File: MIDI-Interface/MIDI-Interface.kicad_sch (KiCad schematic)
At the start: 65 parts, among them J1 Conn_01x06_Pin, J2 Conn_01x01_Pin, J3 Conn_01x01_Pin, J4 Conn_01x14_Pin, J5 Conn_01x14_Pin, SW1 RotaryEncoder_Switch, U1 TL074, U10 Aux_flush, U11 Aux_flush, U12 Aux_flush, U13 Aux_flush, U2 L7806, U3 EL817, U4 TL072, U5 TL074, U6 Aux_flush, U7 Aux_flush, U8 Aux_flush, U9 Aux_flush

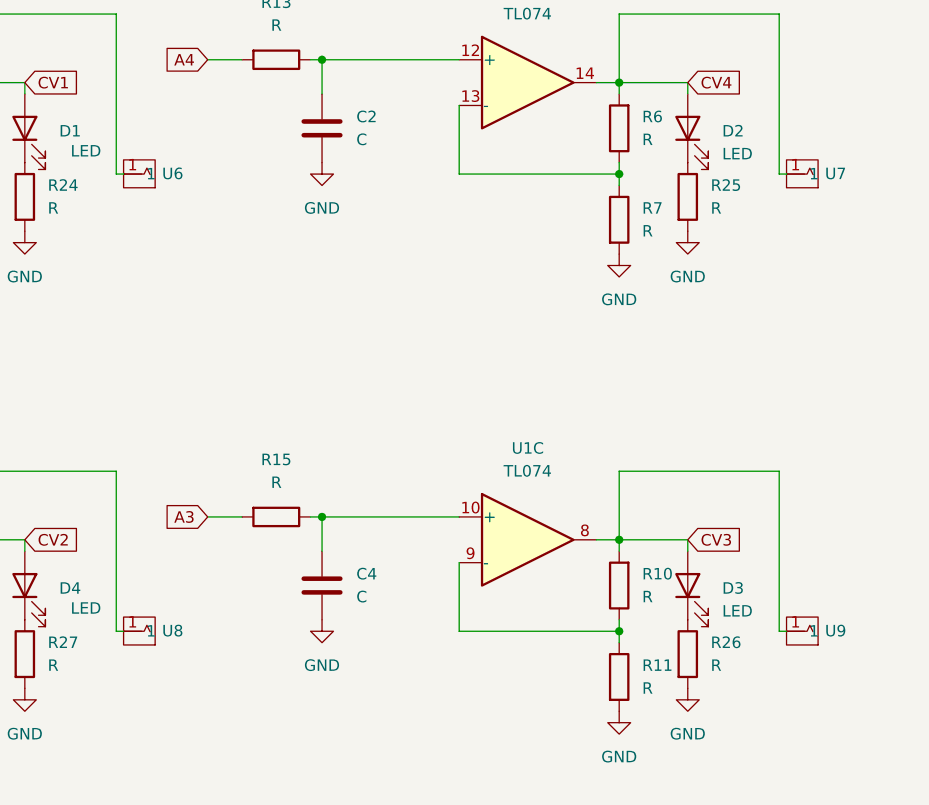
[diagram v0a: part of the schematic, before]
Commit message: Add files via upload
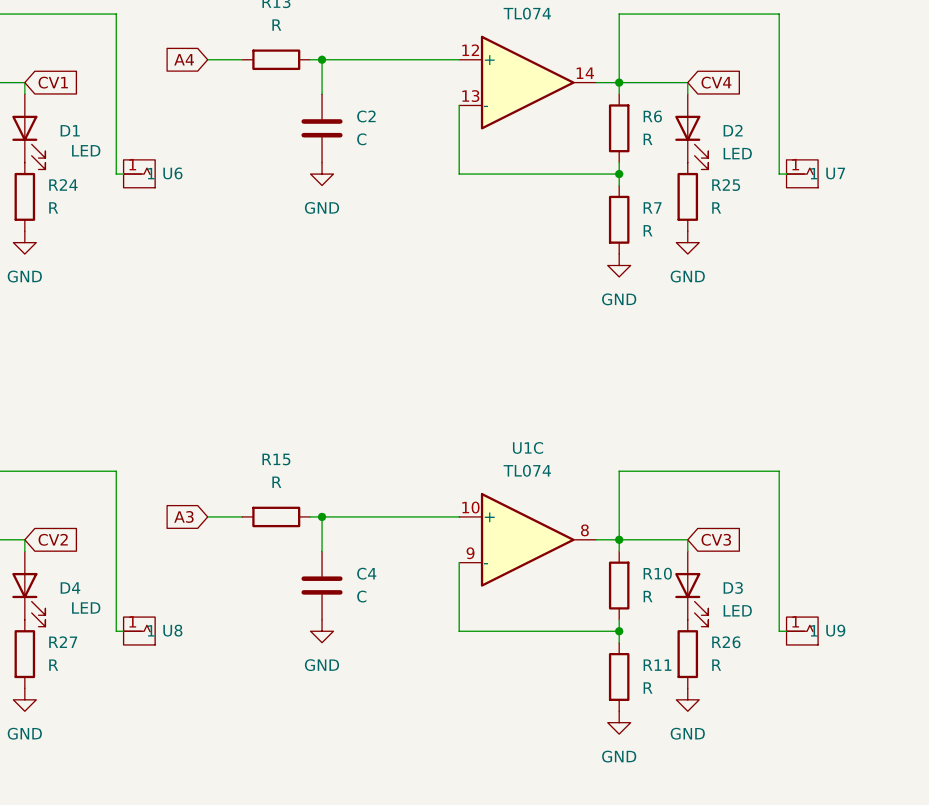
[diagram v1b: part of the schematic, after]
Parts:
- U10, U11, U12, U13, U6, U7, U8, U9: footprint Library:aux_flush -> Library:3mm5 Mono Aux
